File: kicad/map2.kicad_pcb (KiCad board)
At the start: 2 copper layers, 25.4 x 25.4 mm, 16 parts, among them P1 5V, P2 5V, P4 GND, P5 GND, P7 MTG, P8 MTG, Q1 2N2222

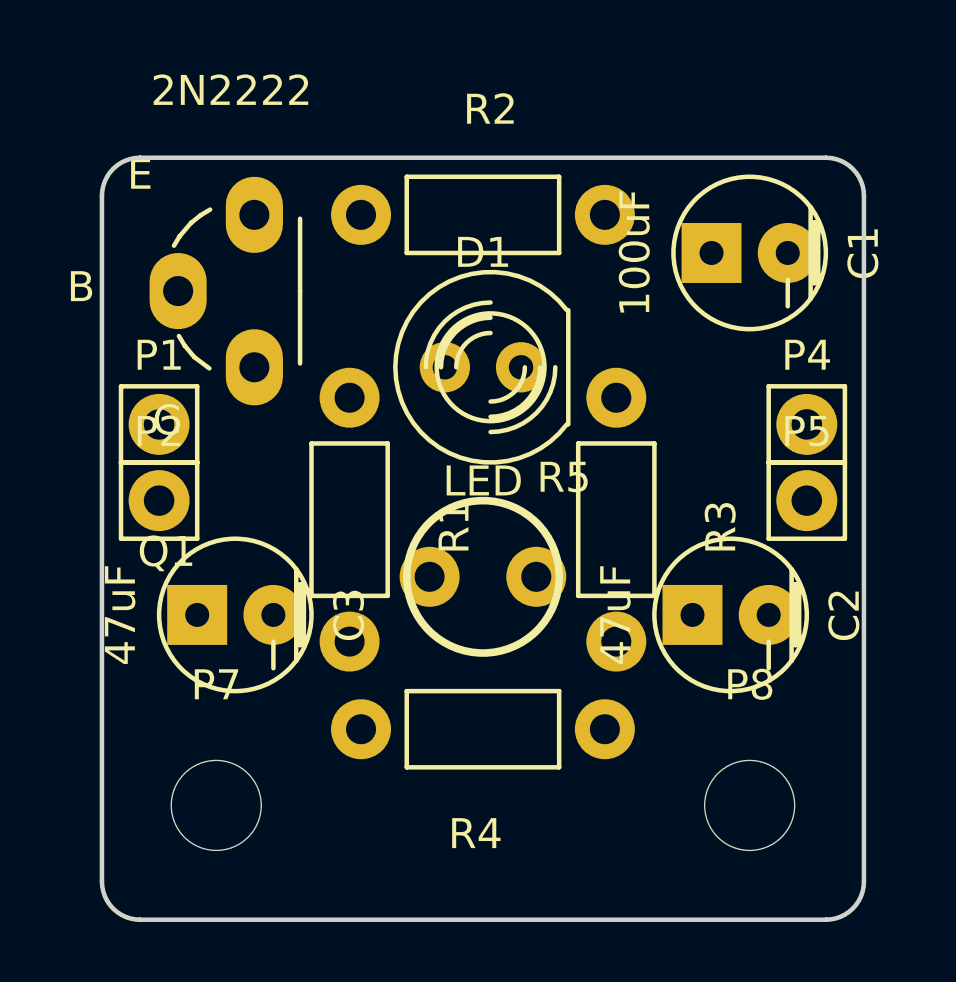
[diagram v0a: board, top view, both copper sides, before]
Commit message: work in progress
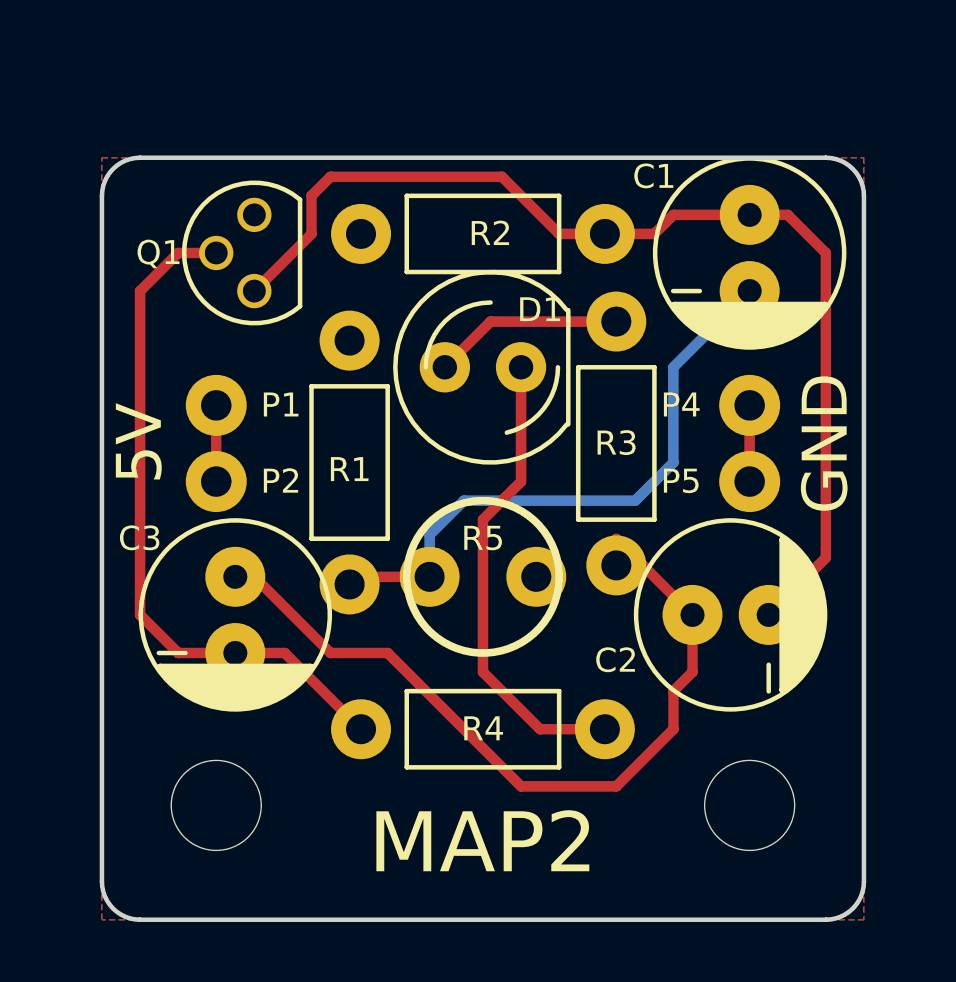
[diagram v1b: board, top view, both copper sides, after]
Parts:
- added P9: LOGO, map2:MA_logo, B.Cu at (127.0, 88.9)
- P1, P2, P4, P5: moved to B.Cu
- Q1: footprint map2:TO-92-Bipolar-rugged-CBE -> map2:TO-92_Molded_Narrow
- moved R3 2.54 mm to (131.4, 90.8)
- moved P1 2.01 mm to (118.1, 89.5), turned to 270 degrees
- moved P4 2.01 mm to (135.9, 89.5), turned to 90 degrees
- moved P2 2.01 mm to (118.1, 92.1), turned to 270 degrees
- moved P5 2.01 mm to (135.9, 92.1), turned to 90 degrees
- moved R1 1.91 mm to (122.6, 91.4)
- moved Q1 1.27 mm to (119.4, 84.5), turned to 90 degrees
- moved R2 0.63 mm to (127.0, 83.8)
- turned C1 to 180 degrees
- turned C3 to 180 degrees
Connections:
- net Net-(BT1-Pad+) renamed /5V
- net Net-(BT1-Pad-) renamed /GND
- net Net-(C1-Pad1) renamed /BASE
- net Net-(C1-Pad2) renamed /LDR
- net Net-(D1-Pad2) renamed /LED
- C3 pad 1: Net-(C3-Pad1) -> Net-(C2-Pad1)
- C3 pad 2: Net-(C2-Pad1) -> /COLL
- Q1 pad 2: Net-(C3-Pad1) -> /COLL
- R4 pad 2: Net-(C3-Pad1) -> /COLL
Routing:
- net /BASE: track 0.00 -> 35.8 mm
- net Net-(C2-Pad1): track 0.00 -> 26.5 mm
- net /COLL: track 0.00 -> 22.8 mm
- net /LDR: track 0.00 -> 20.1 mm
- net /LED: track 0.00 -> 15.5 mm
- net /5V: track 0.00 -> 8.89 mm
- net /GND: track 0.00 -> 2.54 mm
- added copper zone on F.Cu, net /5V
- added copper zone on B.Cu, net /GND
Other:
- net class Default: trace_width 0.25 -> 0.35
- board text added: "5V"
- board text added: "GND"
- board text added: "MAP2"

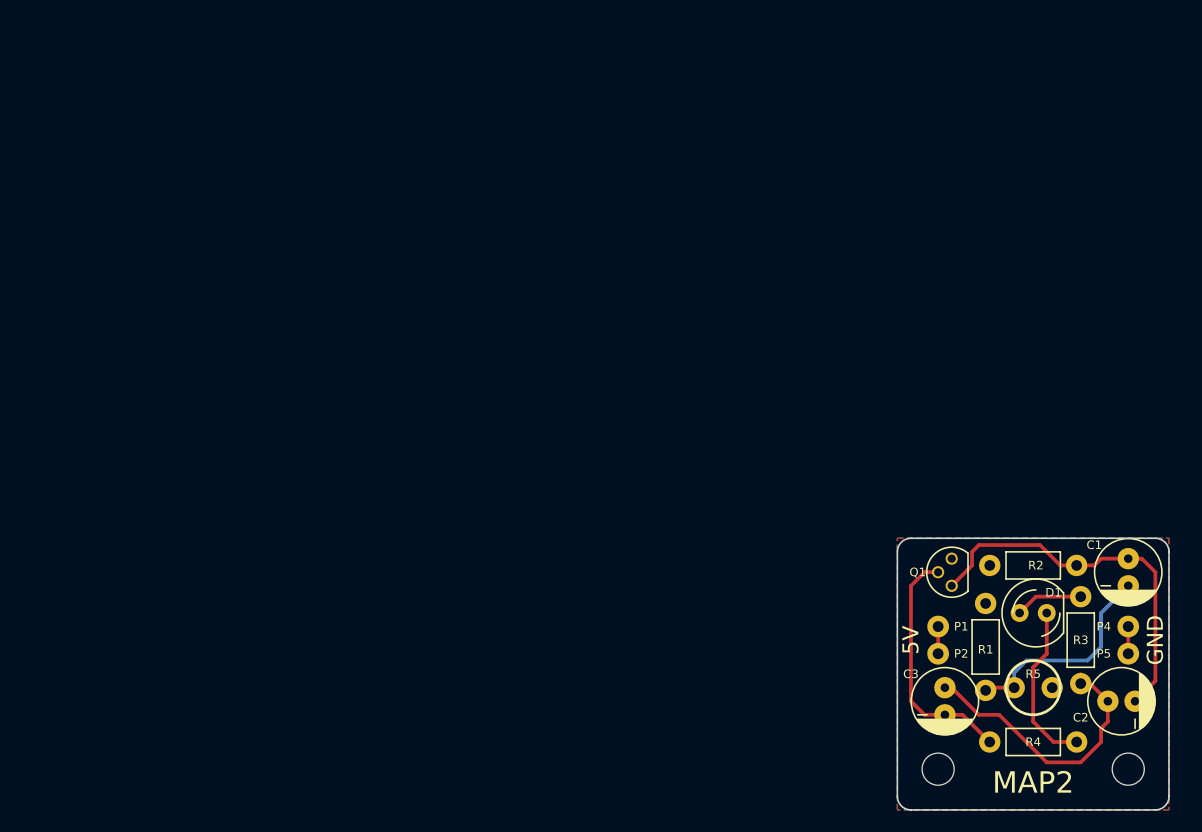
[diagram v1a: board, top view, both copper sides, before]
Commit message: gerbers ready
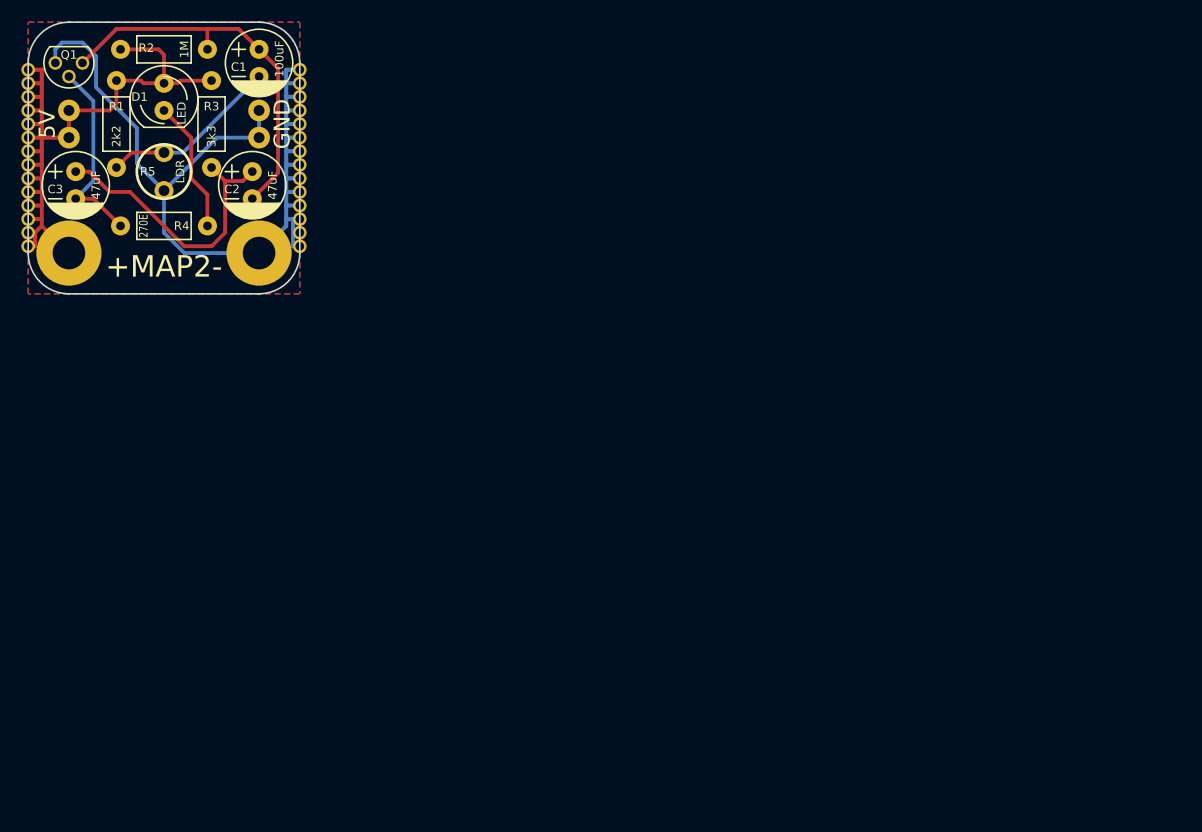
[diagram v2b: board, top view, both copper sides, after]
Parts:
- added REF**11: via, map2:via, F.Cu at (58.4, 37.5)
- added REF**110: via, map2:via, F.Cu at (58.4, 48.9)
- added REF**111: via, map2:via, F.Cu at (58.4, 50.2)
- added REF**1111: via, map2:via, F.Cu at (33.0, 37.5)
- added REF**11110: via, map2:via, F.Cu at (33.0, 48.9)
- added REF**11111: via, map2:via, F.Cu at (33.0, 50.2)
- added REF**11112: via, map2:via, F.Cu at (33.0, 51.4)
- added REF**11113: via, map2:via, F.Cu at (33.0, 52.7)
- added REF**11114: via, map2:via, F.Cu at (33.0, 54.0)
- added REF**1112: via, map2:via, F.Cu at (33.0, 38.7)
- added REF**1113: via, map2:via, F.Cu at (33.0, 40.0)
- added REF**1114: via, map2:via, F.Cu at (33.0, 41.3)
- added REF**1115: via, map2:via, F.Cu at (33.0, 42.5)
- added REF**1116: via, map2:via, F.Cu at (33.0, 43.8)
- added REF**1117: via, map2:via, F.Cu at (33.0, 45.1)
- added REF**1118: via, map2:via, F.Cu at (33.0, 46.4)
- added REF**1119: via, map2:via, F.Cu at (33.0, 47.6)
- added REF**112: via, map2:via, F.Cu at (58.4, 51.4)
- added REF**113: via, map2:via, F.Cu at (58.4, 52.7)
- added REF**114: via, map2:via, F.Cu at (58.4, 54.0)
- added REF**12: via, map2:via, F.Cu at (58.4, 38.7)
- added REF**13: via, map2:via, F.Cu at (58.4, 40.0)
- added REF**14: via, map2:via, F.Cu at (58.4, 41.3)
- added REF**15: via, map2:via, F.Cu at (58.4, 42.5)
- added REF**16: via, map2:via, F.Cu at (58.4, 43.8)
- added REF**17: via, map2:via, F.Cu at (58.4, 45.1)
- added REF**18: via, map2:via, F.Cu at (58.4, 46.4)
- added REF**19: via, map2:via, F.Cu at (58.4, 47.6)
- P7, P8: footprint map2:MountingHole_3mm -> map2:MTG_3mm
- R5: value R_photo -> LDR
- moved P8 110.2 mm to (36.8, 54.6)
- moved Q1 95.3 mm to (36.8, 36.8), turned to 180 degrees
- moved R1 94.9 mm to (41.3, 42.5)
- moved C2 94.5 mm to (54.0, 48.3), turned to 180 degrees
- moved C3 94.5 mm to (37.5, 48.3)
- moved D1 94.5 mm to (45.7, 40.0), turned to 270 degrees
- moved P1 94.5 mm to (36.8, 41.3)
- moved P2 94.5 mm to (36.8, 43.8)
- moved R2 94.5 mm to (45.7, 35.6)
- moved R3 94.5 mm to (50.2, 42.5)
- moved R4 94.5 mm to (45.7, 52.1)
- moved R5 94.5 mm to (45.7, 47.0), turned to 270 degrees
- moved P4 94.5 mm to (54.6, 41.3)
- moved P5 94.5 mm to (54.6, 43.8)
- moved C1 94.2 mm to (54.6, 36.8)
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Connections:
- P7 pad 1: (no net) -> /GND
- P8 pad 1: (no net) -> /5V
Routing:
- net /GND: track 2.54 -> 85.4 mm
- net /5V: track 8.89 -> 64.9 mm
- net /COLL: track 22.8 -> 18.3 mm
- net /LDR: track 20.1 -> 16.9 mm
- net /LED: track 15.5 -> 12.5 mm
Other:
- outline, holes or cut-outs redrawn
- net class Default: clearance 0.2 -> 0.1905; trace_width 0.35 -> 0.381; via_dia 0.6 -> 0.762; via_drill 0.4 -> 0.508
- rule trace_clearance: 0.2 -> 0.1905
- rule trace_min: 0.2 -> 0.1905
- rule via_min_drill: 0.3 -> 0.508
- rule via_min_size: 0.4 -> 0.762
- board text added: "+MAP2-"
- board text added: "makersasylum.com"
- board text removed: "MAP2"
